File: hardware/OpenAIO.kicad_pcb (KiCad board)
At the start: 8 copper layers, 35 x 35 mm, 341 parts, among them J15 5V, J16 5V, J17 5V, J18 5V, J20 5V, J21 5V, J23 5V, J24 5V, J25 5V, J26 5V, J27 5V, J28 5V, J29 5V, J30 5V, J31 5V, J32 5V, J33 5V, J34 5V, J35 5V, J37 5V, J38 5V, J39 5V, J40 5V, J41 5V, J42 5V, J43 5V, J44 5V, J45 5V, J48 5V, J49 5V, J50 5V, J51 5V, J52 5V, J53 5V, J54 5V, J55 5V, Q1 AP1606, Q10 DOY180N03T, Q11 DOY180N03T, Q12 DOY180N03T, Q13 DOY180N03T, Q14 DOY180N03T, Q15 DOY180N03T, Q16 DOY180N03T, Q17 DOY180N03T, Q18 DOY180N03T, Q19 DOY180N03T, Q2 AP1606, Q20 DOY180N03T, Q21 DOY180N03T, Q22 DOY180N03T, Q23 DOY180N03T, Q24 DOY180N03T, Q25 DOY180N03T, Q26 DOY180N03T, Q3 DOY180N03T, Q4 DOY180N03T, Q5 DOY180N03T, Q6 DOY180N03T, Q7 DOY180N03T, Q8 DOY180N03T, Q9 DOY180N03T, U1 TS2306A 240GF MSM 9_C2976675, U10 COS8051SOT, U11 TLV7031DPWR, U12 SM06B-SRSS-TB(LF)(SN), U13 AT32F421G8U7, U14 NSG2065Q, U15 AT32F421G8U7, U16 NSG2065Q, U17 AT32F421G8U7, U18 NSG2065Q, U19 AT32F421G8U7, U2 RP2354A, U20 NSG2065Q, U21 SX1281IMLTRT, U22 ESP32-C3, U24 AIO_outline, U25 INA186A3IDCKR, U26 BMP580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

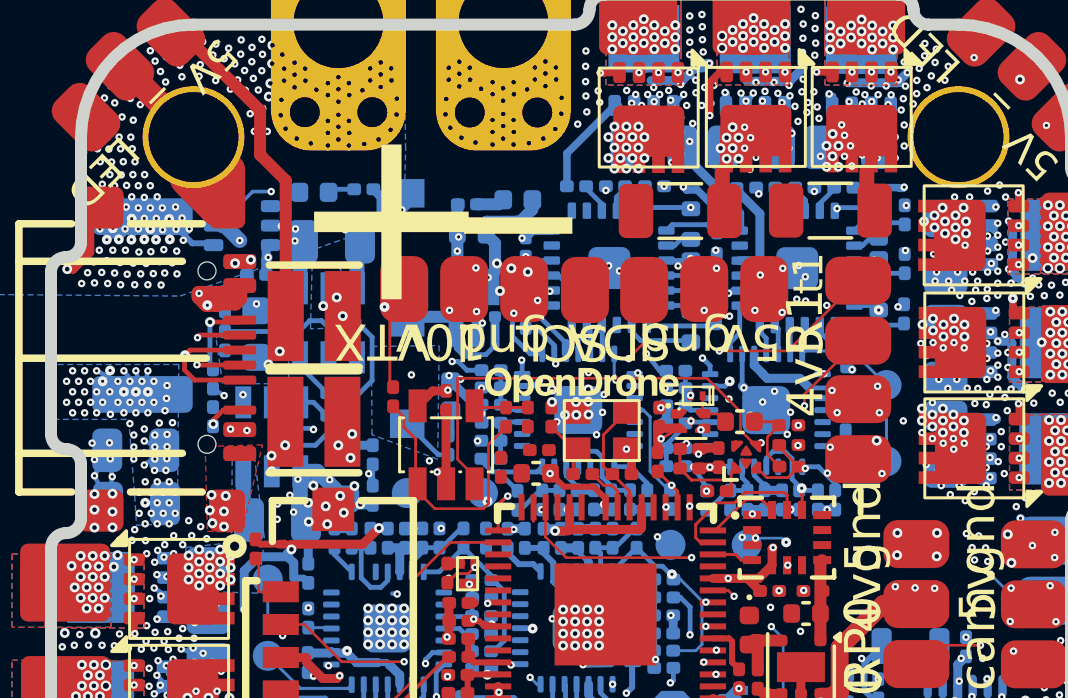
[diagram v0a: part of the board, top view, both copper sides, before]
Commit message: Owner: routing in progress
Co-Authored-By: Claude Opus 5.5 <noreply@anthropic.com>
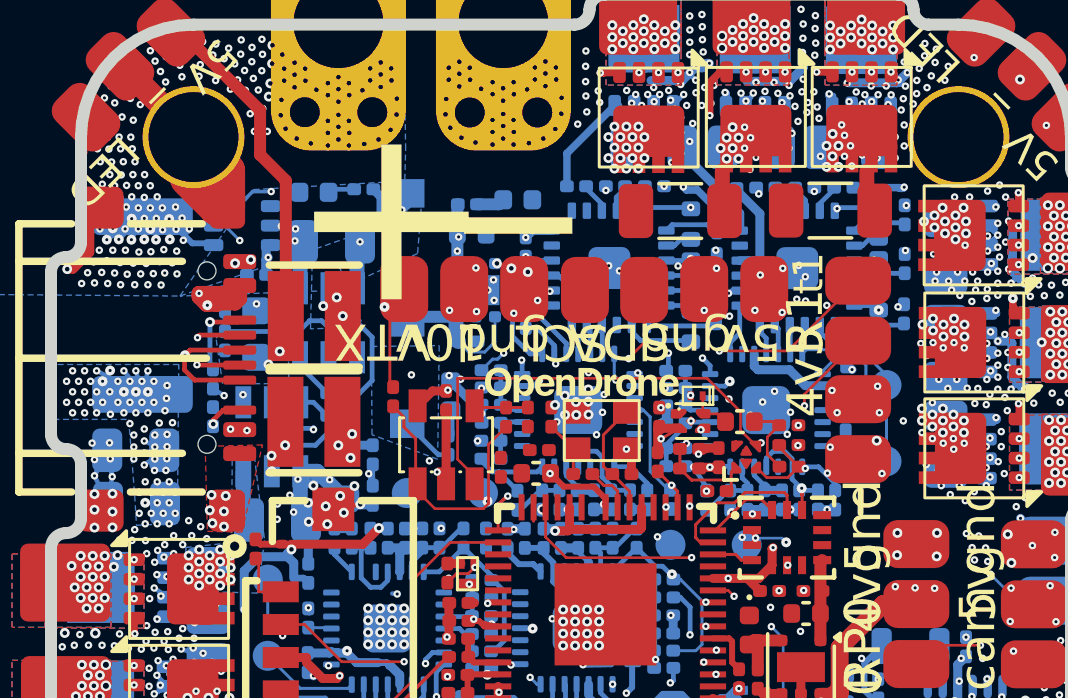
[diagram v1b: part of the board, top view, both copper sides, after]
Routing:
- net +5V: track 86.7 -> 57.3 mm
- net +3.3V: track 105.4 -> 84.5 mm
- net BUZZER-: track 20.7 -> 2.38 mm
- net GND: track 148.1 -> 132.0 mm, vias 905 -> 908
- net +10V: track 66.2 -> 50.8 mm
- net /3A: track 1.15 -> 10.4 mm, vias 23 -> 24
- net /Pads/PU0RX: track 11.4 -> 2.52 mm
- net /4A: track 8.47 -> 17.3 mm, vias 22 -> 23
- net +5V_USB: track 21.1 -> 13.1 mm
- net SPI0.MOSI: track 13.7 -> 6.77 mm
- net /4C: track 24.1 -> 18.5 mm
- net +BATT: track 19.8 -> 23.0 mm
- net /Pads/I2C0.SDA: track 18.3 -> 16.1 mm
- net /3B: track 20.8 -> 19.5 mm
- net /3C: track 20.2 -> 19.1 mm
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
